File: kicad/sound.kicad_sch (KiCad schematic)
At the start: 17 parts, among them J4 Speaker, U11 74HC02, U16 74HC00, U17 LM386, U3 PSG_AY-3-8912

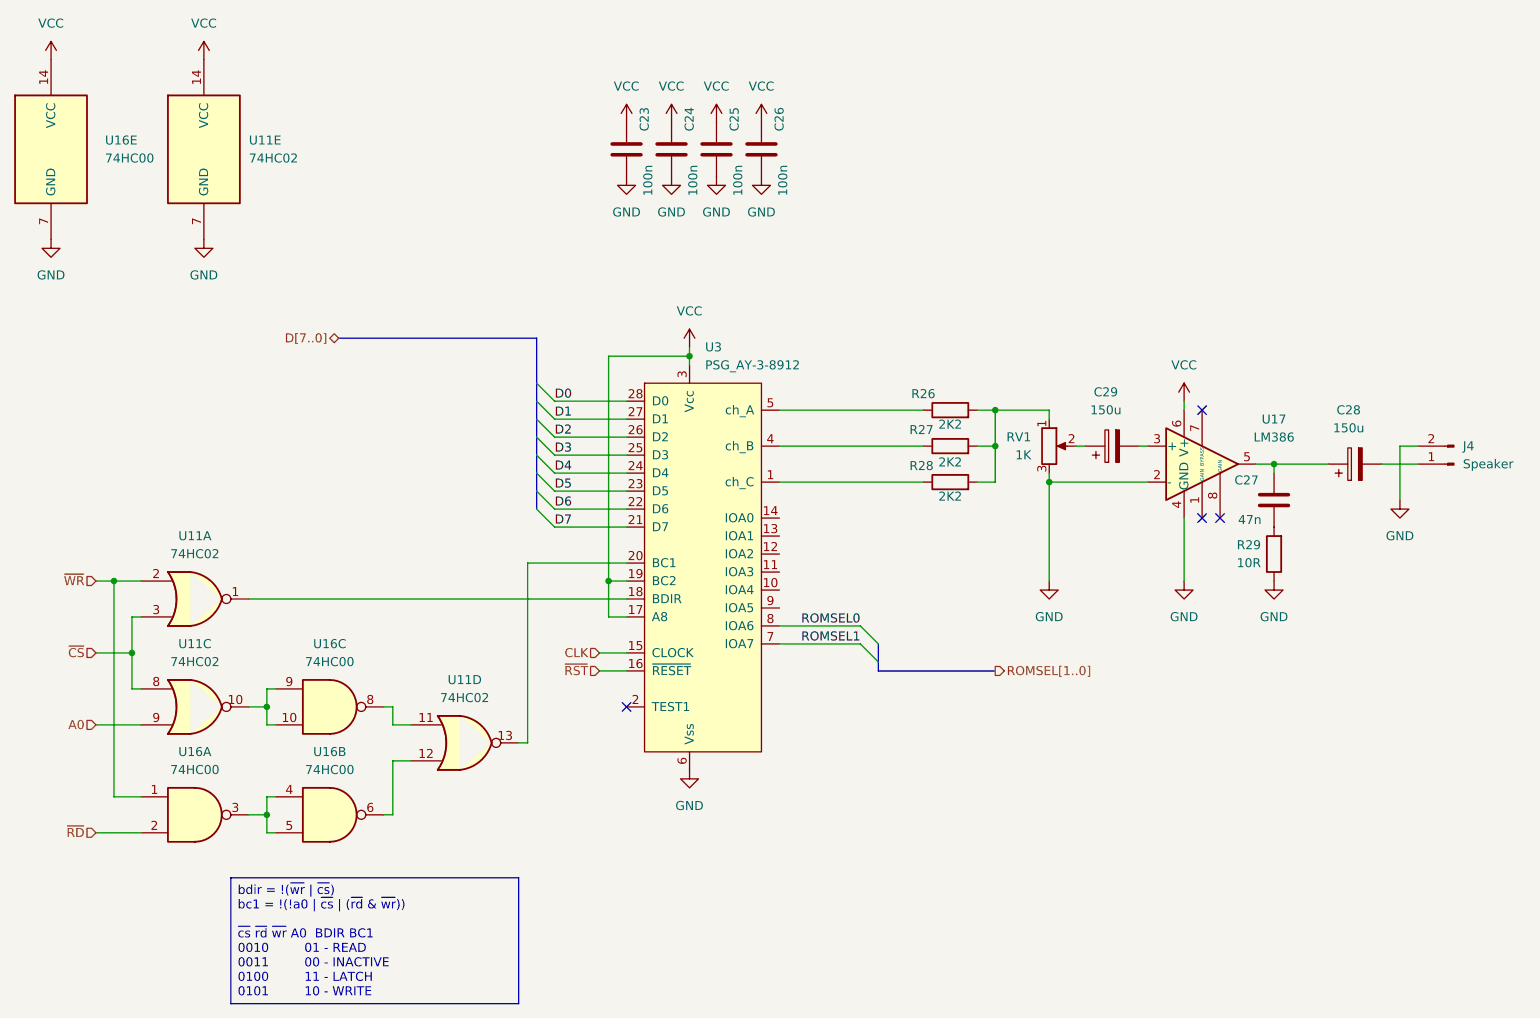
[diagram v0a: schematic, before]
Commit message: hw: finish schematic, start routing
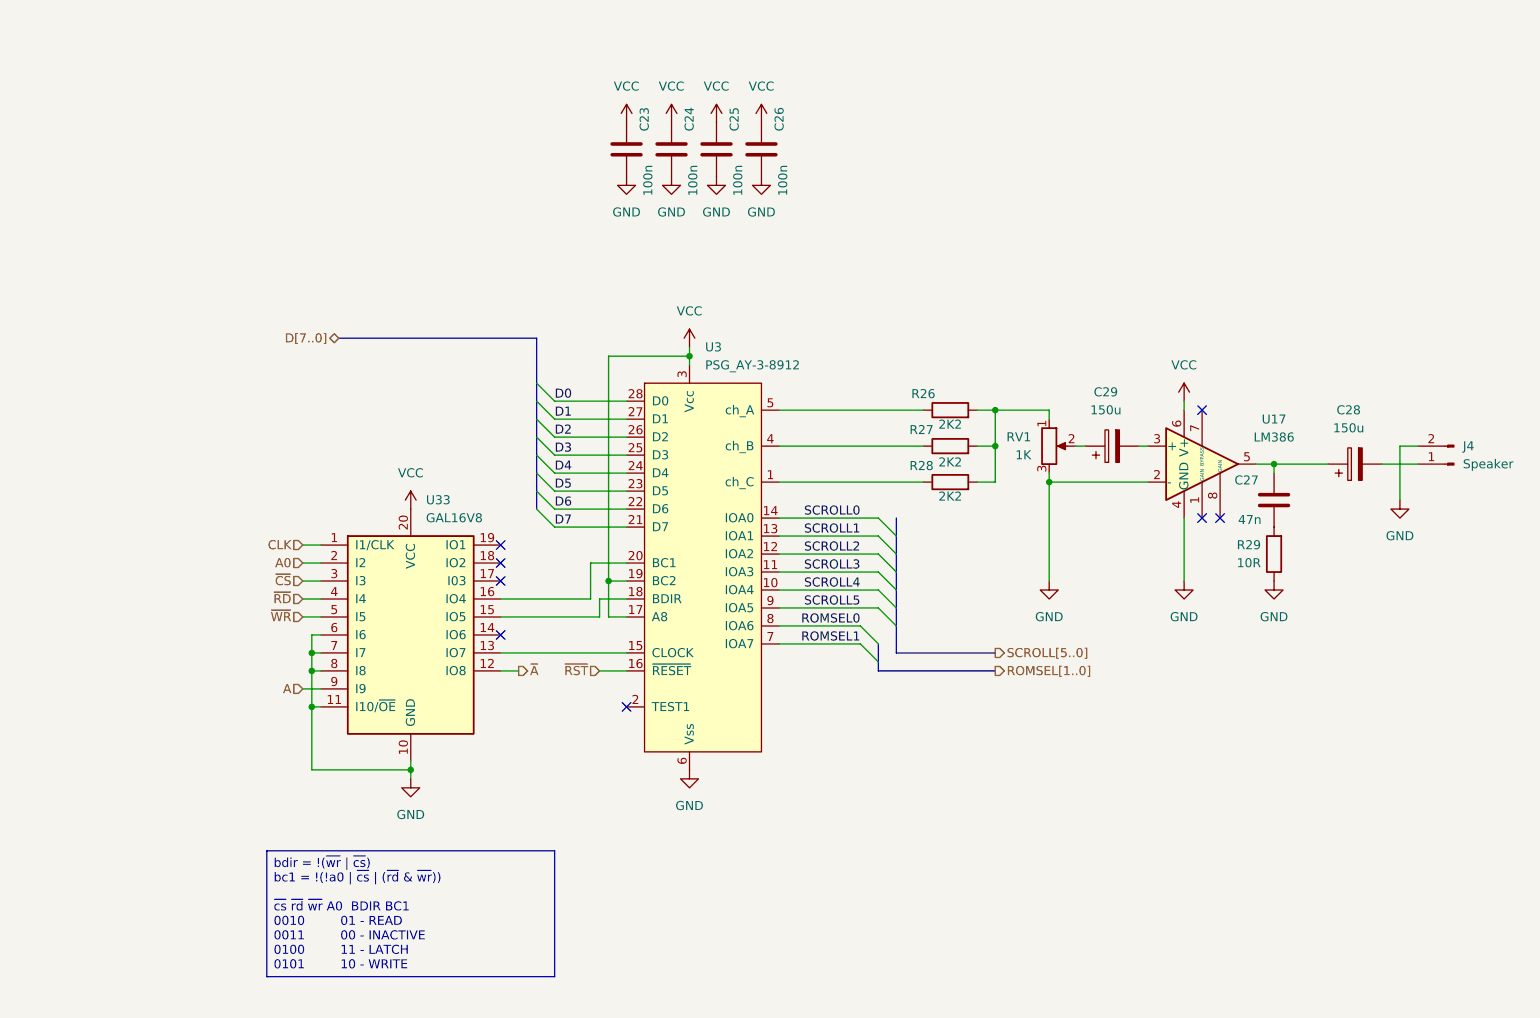
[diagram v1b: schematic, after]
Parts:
- removed U11: 74HC02, Package_DIP:DIP-14_W7.62mm, symbol 74xx:74HC02
- removed U16: 74HC00, Package_DIP:DIP-14_W7.62mm, symbol 74xx:74HC00
- added U33: GAL16V8, Package_DIP:DIP-20_W7.62mm, symbol Logic_Programmable:GAL16V8
- J4: footprint Connector_PinHeader_2.54mm:PinHeader_1x02_P2.54mm_Horizontal -> Connector_PinHeader_2.54mm:PinHeader_1x02_P2.54mm_Vertical
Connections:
- net A0: now also U33.2 (I2)
- net CLK: now also U33.1 (I1/CLK); no longer U3.15 (CLOCK)
- net GND: now also U33.10 (GND), U33.11 (I10/~{OE}), U33.6 (I6), U33.7 (I7), U33.8 (I8)
- net VCC: now also U33.20 (VCC)
- net ~{CS}: now also U33.3 (I3)
- net ~{RD}: now also U33.4 (I4)
- net ~{WR}: now also U33.5 (I5)
- net at U3.18 (BDIR): now also U33.15 (IO5)
- net SCROLL4: now reaches U3.10 (IOA4)
- net SCROLL3: now reaches U3.11 (IOA3)
- net SCROLL2: now reaches U3.12 (IOA2)
- net SCROLL1: now reaches U3.13 (IOA1)
- net SCROLL0: now reaches U3.14 (IOA0)
- net at U3.20 (BC1): now also U33.16 (IO4)
- net SCROLL5: now reaches U3.9 (IOA5)
- new net: U3.15 (CLOCK), U33.13 (IO7)
- new net A: U33.9 (I9)
- new net ~{A}: U33.12 (IO8)
- no-connect marks 4 -> 8
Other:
- company: (none) -> A.K.
- title: (none) -> Sound
